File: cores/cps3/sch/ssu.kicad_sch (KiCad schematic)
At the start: 1 part

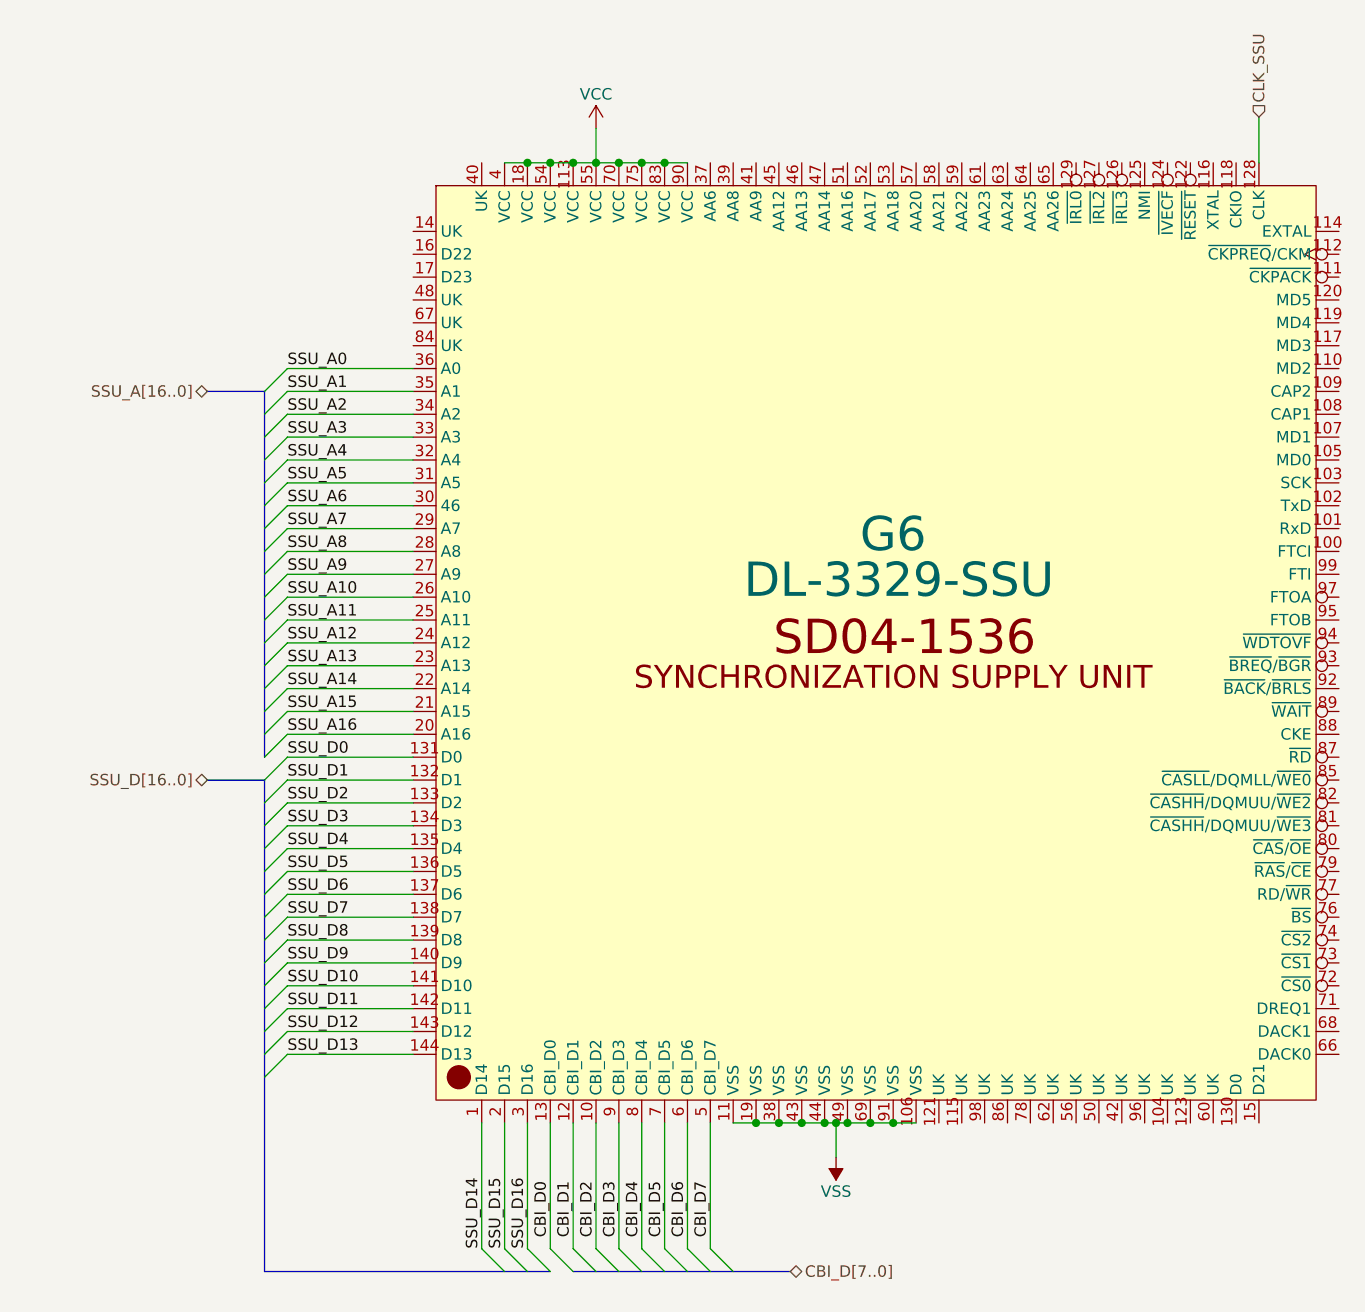
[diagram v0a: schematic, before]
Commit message: update6_cps
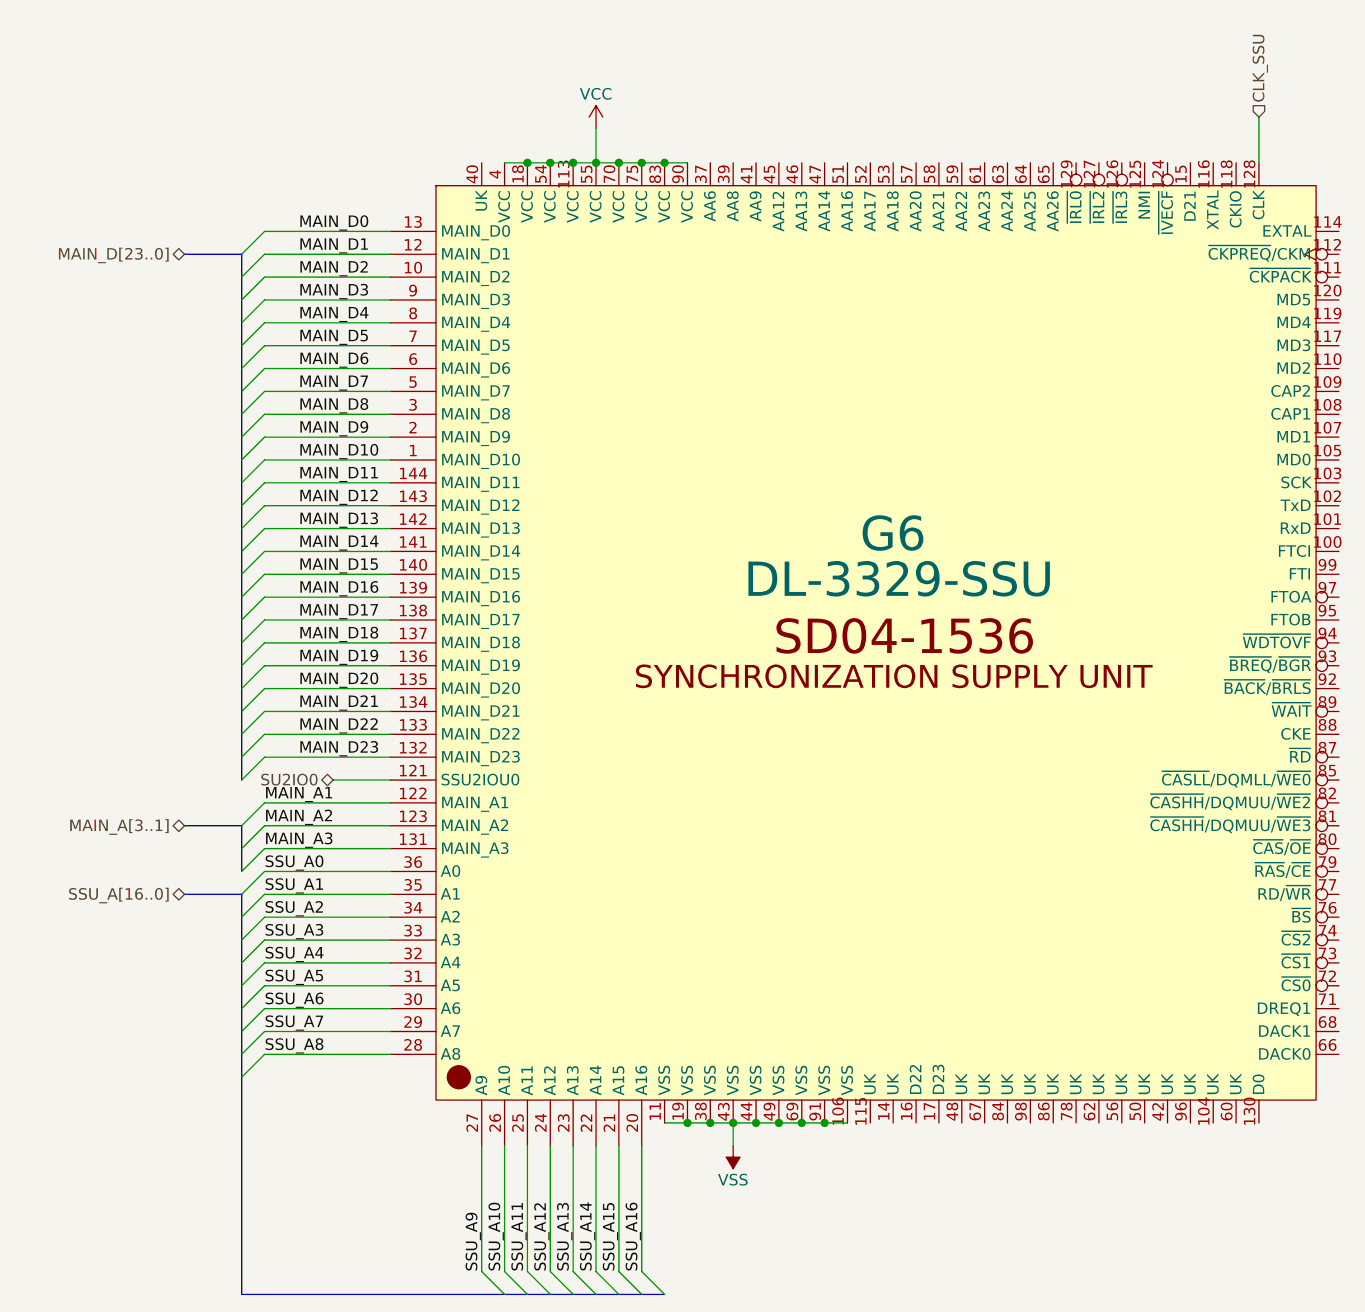
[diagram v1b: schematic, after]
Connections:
- net SU2IO0: now reaches G6.121 (SSU2IOU0)
- net MAIN_A1: now reaches G6.122 (MAIN_A1)
- net MAIN_A2: now reaches G6.123 (MAIN_A2)
- net CBI_D0 renamed MAIN_D0
- net CBI_D1 renamed MAIN_D1
- net CBI_D2 renamed MAIN_D2
- net CBI_D3 renamed MAIN_D3
- net CBI_D4 renamed MAIN_D4
- net CBI_D5 renamed MAIN_D5
- net CBI_D6 renamed MAIN_D6
- net CBI_D7 renamed MAIN_D7
- net SSU_D0 renamed MAIN_A3
- net SSU_D1 renamed MAIN_D23
- net SSU_D10 renamed MAIN_D14
- net SSU_D11 renamed MAIN_D13
- net SSU_D12 renamed MAIN_D12
- net SSU_D13 renamed MAIN_D11
- net SSU_D14 renamed MAIN_D10
- net SSU_D15 renamed MAIN_D9
- net SSU_D16 renamed MAIN_D8
- net SSU_D2 renamed MAIN_D22
- net SSU_D3 renamed MAIN_D21
- net SSU_D4 renamed MAIN_D20
- net SSU_D5 renamed MAIN_D19
- net SSU_D6 renamed MAIN_D18
- net SSU_D7 renamed MAIN_D17
- net SSU_D8 renamed MAIN_D16
- net SSU_D9 renamed MAIN_D15
